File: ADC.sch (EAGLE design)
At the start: 368 parts, among them IC1 AD8221ARZ, IC10 AD8605ARTZ, IC11 AD8221ARZ, IC12 TLC2254ID, IC13 AD8605ARTZ, IC14 AD8221ARZ, IC15 TLC2254ID, IC16 AD8605ARTZ, IC17 AD8221ARZ, IC18 TLC2254ID, IC19 AD8605ARTZ, IC2 TLC2254ID, IC20 AD8221ARZ, IC21 TLC2254ID, IC22 AD8605ARTZ, IC23 AD8221ARZ, IC24 TLC2254ID, IC25 AD8605ARTZ, IC26 AD8221ARZ, IC27 TLC2254ID, IC28 AD8605ARTZ, IC3 ADS1256IDBT, IC4 AD8605ARTZ, IC5 MCP170333MB, IC6 ADUM1402ARWZ, IC7 REF3125AIDBZT, IC8 AD8221ARZ, IC9 TLC2254ID, Q1 8MHz

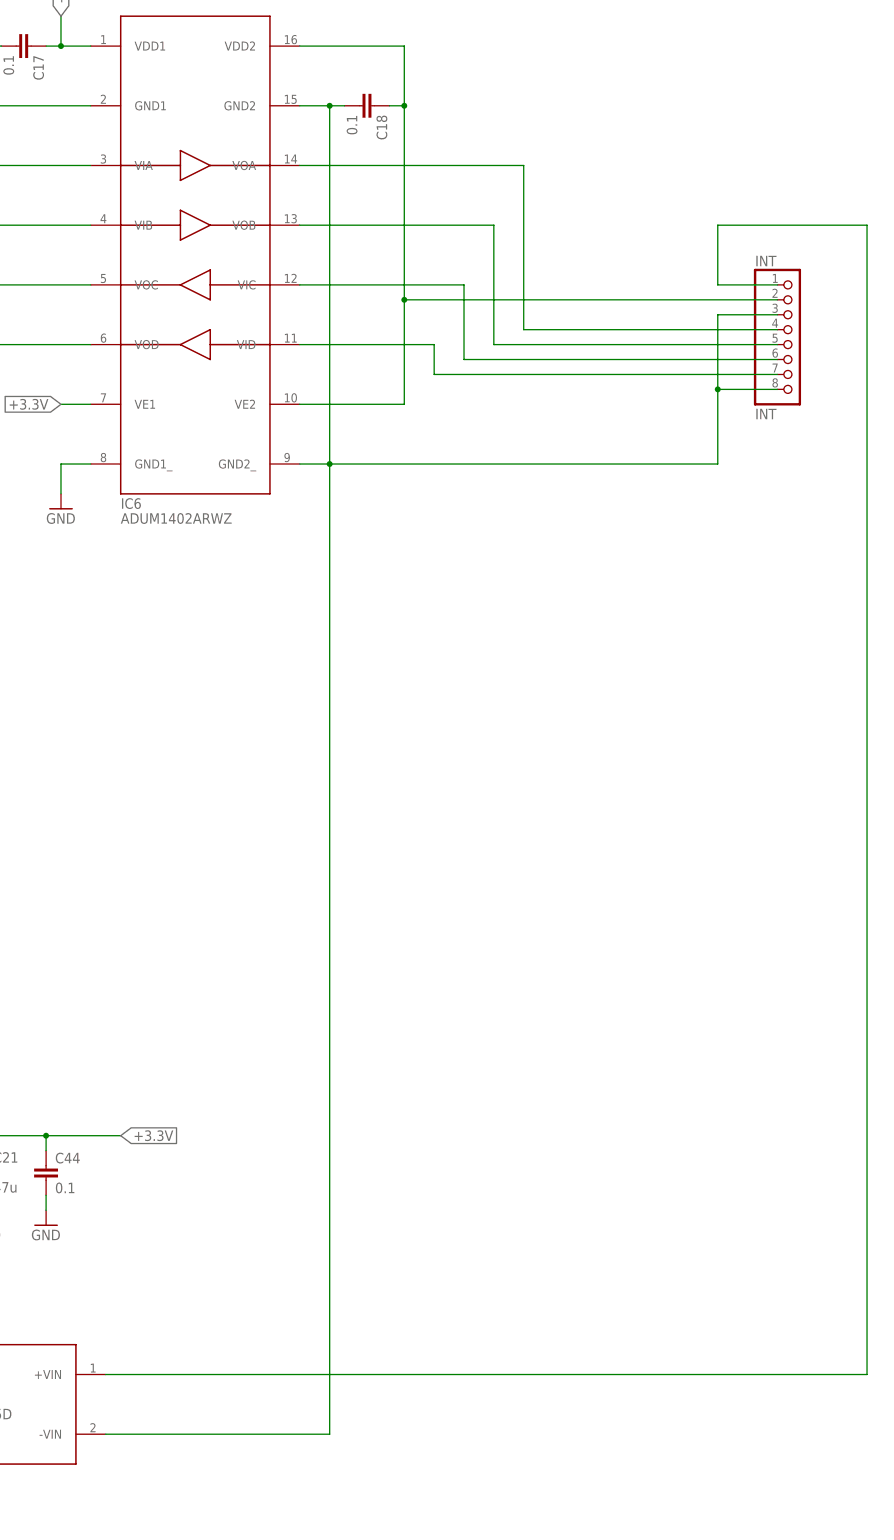
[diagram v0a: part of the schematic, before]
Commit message: Latest modification for all-in-one board
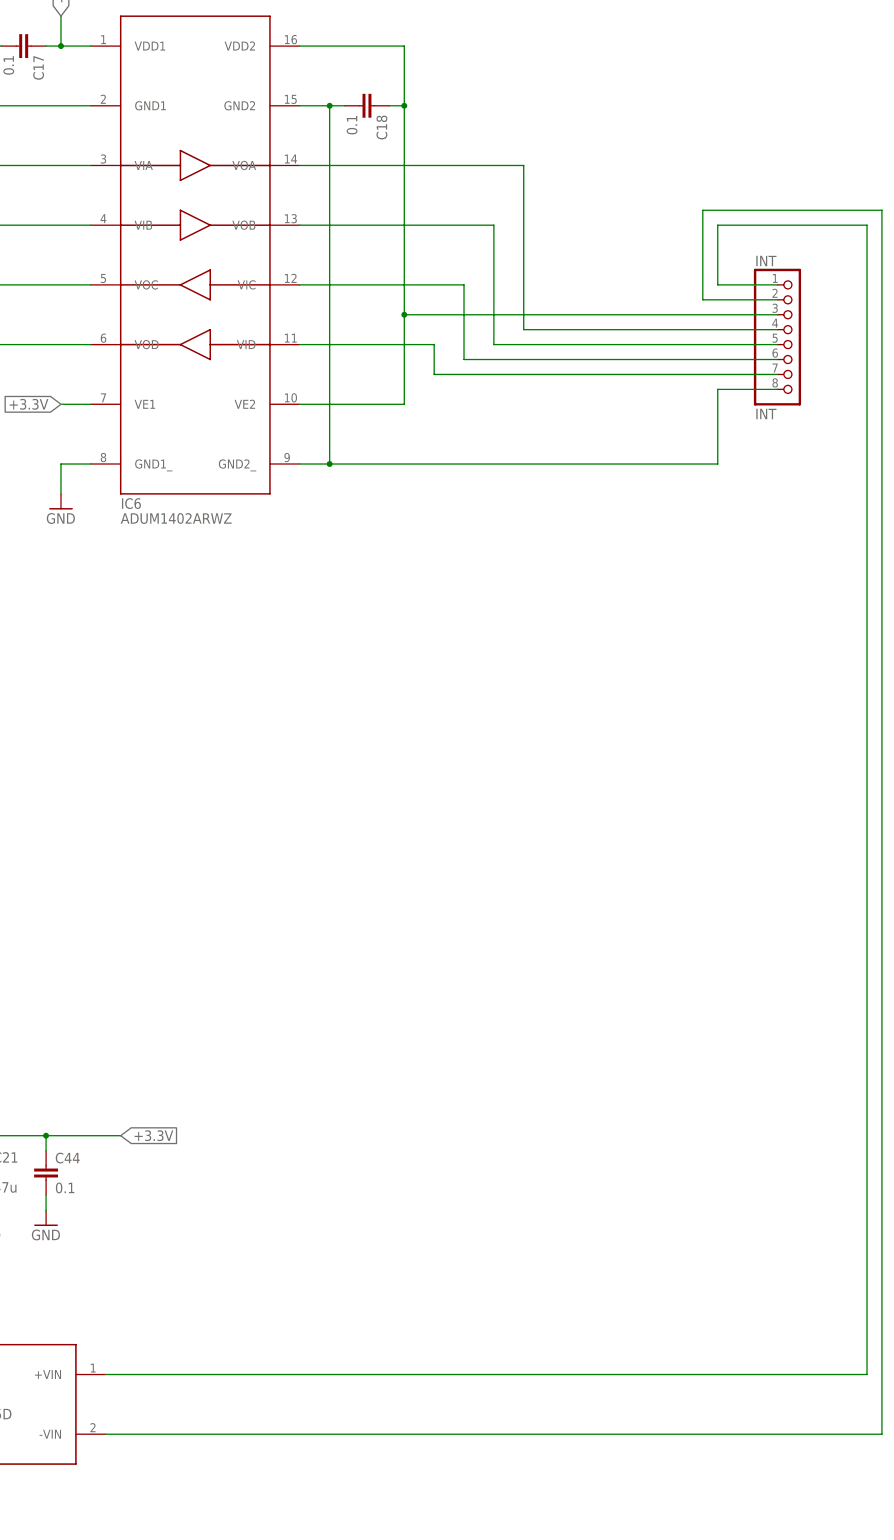
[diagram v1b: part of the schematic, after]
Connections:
- new net N$207: G1.-VIN, INT.2
- net N$37: no longer G1.-VIN, INT.3
- net N$38: now also INT.3; no longer INT.2
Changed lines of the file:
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@@
 <net name="N$37" class="0">
 <segment>
-<wire x1="695.96" y1="-167.64" x2="695.96" y2="-2.54" width="0.1524" layer="91"/>
 <pinref part="IC6" gate="G$1" pin="GND2_"/>
 <wire x1="695.96" y1="-2.54" x2="690.88" y2="-2.54" width="0.1524" layer="91"/>
@@
 <wire x1="695.96" y1="58.42" x2="698.5" y2="58.42" width="0.1524" layer="91"/>
 <junction x="695.96" y="58.42"/>
-<pinref part="INT" gate="A" pin="3"/>
-<wire x1="772.16" y1="22.86" x2="762" y2="22.86" width="0.1524" layer="91"/>
-<wire x1="762" y1="22.86" x2="762" y2="10.16" width="0.1524" layer="91"/>
 <pinref part="INT" gate="A" pin="8"/>
 <wire x1="762" y1="10.16" x2="772.16" y2="10.16" width="0.1524" layer="91"/>
 <wire x1="695.96" y1="-2.54" x2="762" y2="-2.54" width="0.1524" layer="91"/>
 <wire x1="762" y1="-2.54" x2="762" y2="10.16" width="0.1524" layer="91"/>
-<junction x="762" y="10.16"/>
-<pinref part="G1" gate="G$1" pin="-VIN"/>
-<wire x1="657.86" y1="-167.64" x2="695.96" y2="-167.64" width="0.1524" layer="91"/>
 </segment>
 </net>
@@
 <pinref part="IC6" gate="G$1" pin="VE2"/>
 <wire x1="690.88" y1="7.62" x2="708.66" y2="7.62" width="0.1524" layer="91"/>
-<wire x1="708.66" y1="7.62" x2="708.66" y2="25.4" width="0.1524" layer="91"/>
 <pinref part="IC6" gate="G$1" pin="VDD2"/>
-<wire x1="708.66" y1="25.4" x2="708.66" y2="58.42" width="0.1524" layer="91"/>
+<wire x1="708.66" y1="7.62" x2="708.66" y2="22.86" width="0.1524" layer="91"/>
+<wire x1="708.66" y1="22.86" x2="708.66" y2="58.42" width="0.1524" layer="91"/>
 <wire x1="708.66" y1="58.42" x2="708.66" y2="68.58" width="0.1524" layer="91"/>
 <wire x1="708.66" y1="68.58" x2="690.88" y2="68.58" width="0.1524" layer="91"/>
@@
 <wire x1="706.12" y1="58.42" x2="708.66" y2="58.42" width="0.1524" layer="91"/>
 <junction x="708.66" y="58.42"/>
-<pinref part="INT" gate="A" pin="2"/>
-<wire x1="772.16" y1="25.4" x2="708.66" y2="25.4" width="0.1524" layer="91"/>
-<junction x="708.66" y="25.4"/>
+<pinref part="INT" gate="A" pin="3"/>
+<wire x1="772.16" y1="22.86" x2="708.66" y2="22.86" width="0.1524" layer="91"/>
+<junction x="708.66" y="22.86"/>
 </segment>
 </net>
@@
 </segment>
 </net>
+<net name="N$207" class="0">
+<segment>
+<pinref part="G1" gate="G$1" pin="-VIN"/>
+<wire x1="657.86" y1="-167.64" x2="789.94" y2="-167.64" width="0.1524" layer="91"/>
+<wire x1="789.94" y1="-167.64" x2="789.94" y2="40.64" width="0.1524" layer="91"/>
+<wire x1="789.94" y1="40.64" x2="759.46" y2="40.64" width="0.1524" layer="91"/>
+<wire x1="759.46" y1="40.64" x2="759.46" y2="25.4" width="0.1524" layer="91"/>
+<pinref part="INT" gate="A" pin="2"/>
+<wire x1="759.46" y1="25.4" x2="772.16" y2="25.4" width="0.1524" layer="91"/>
+</segment>
+</net>
